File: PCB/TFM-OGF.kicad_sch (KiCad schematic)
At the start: 16 parts, among them J1 Alimentación, J2 CAN, J3 Jumper CAN, J4 Jumper CAN, U1 SN65HVD230, U2 SN65HVD230

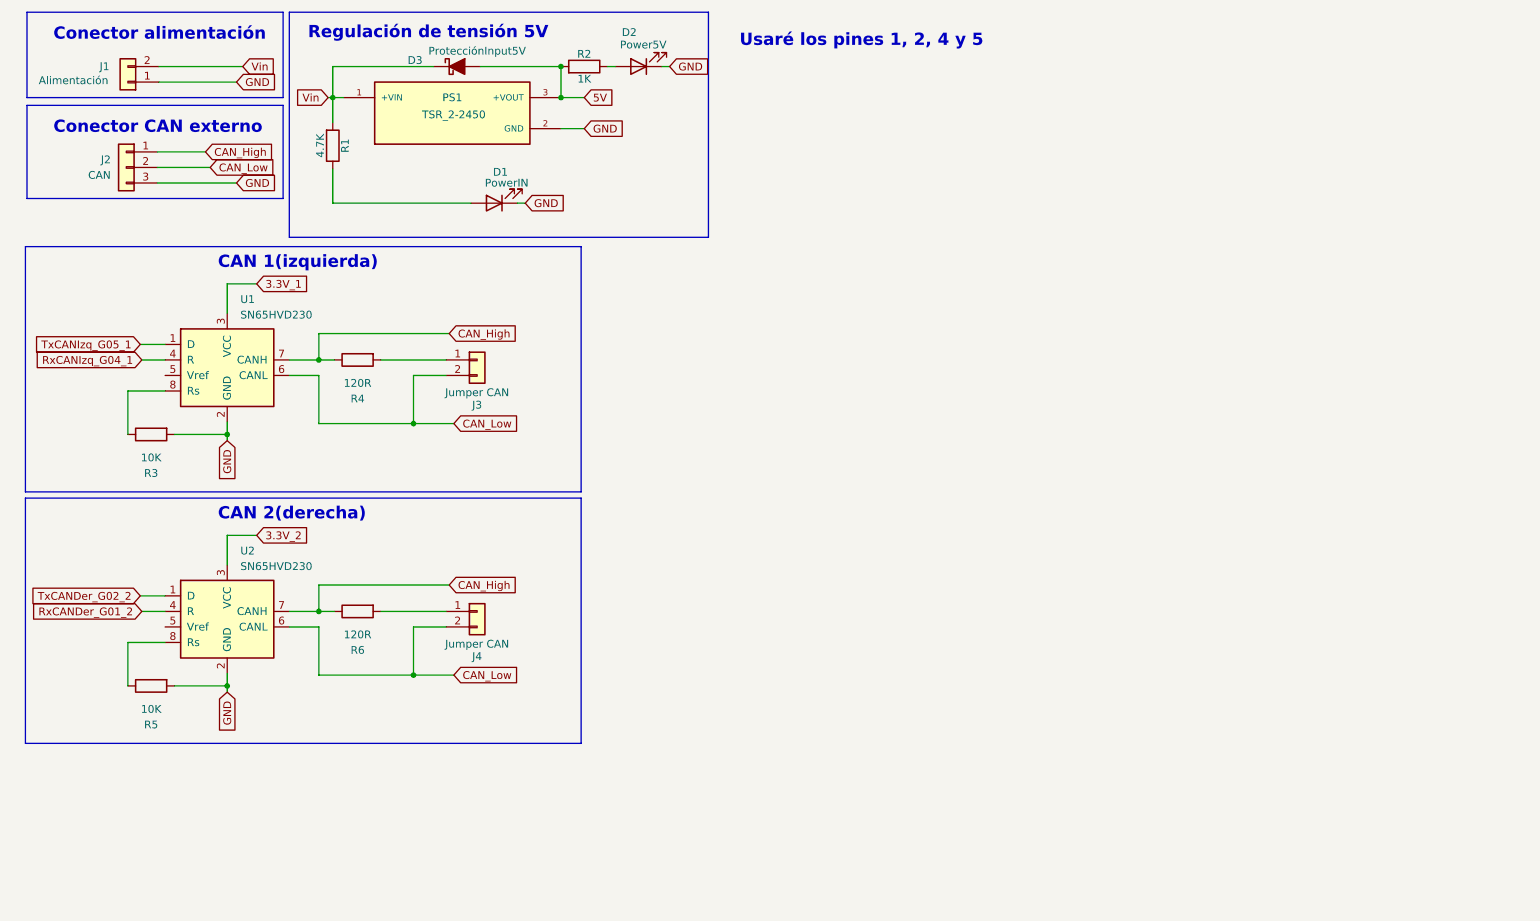
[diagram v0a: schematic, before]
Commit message: Finalizo esquemático, usaré medidas y caja de BrakeCAN
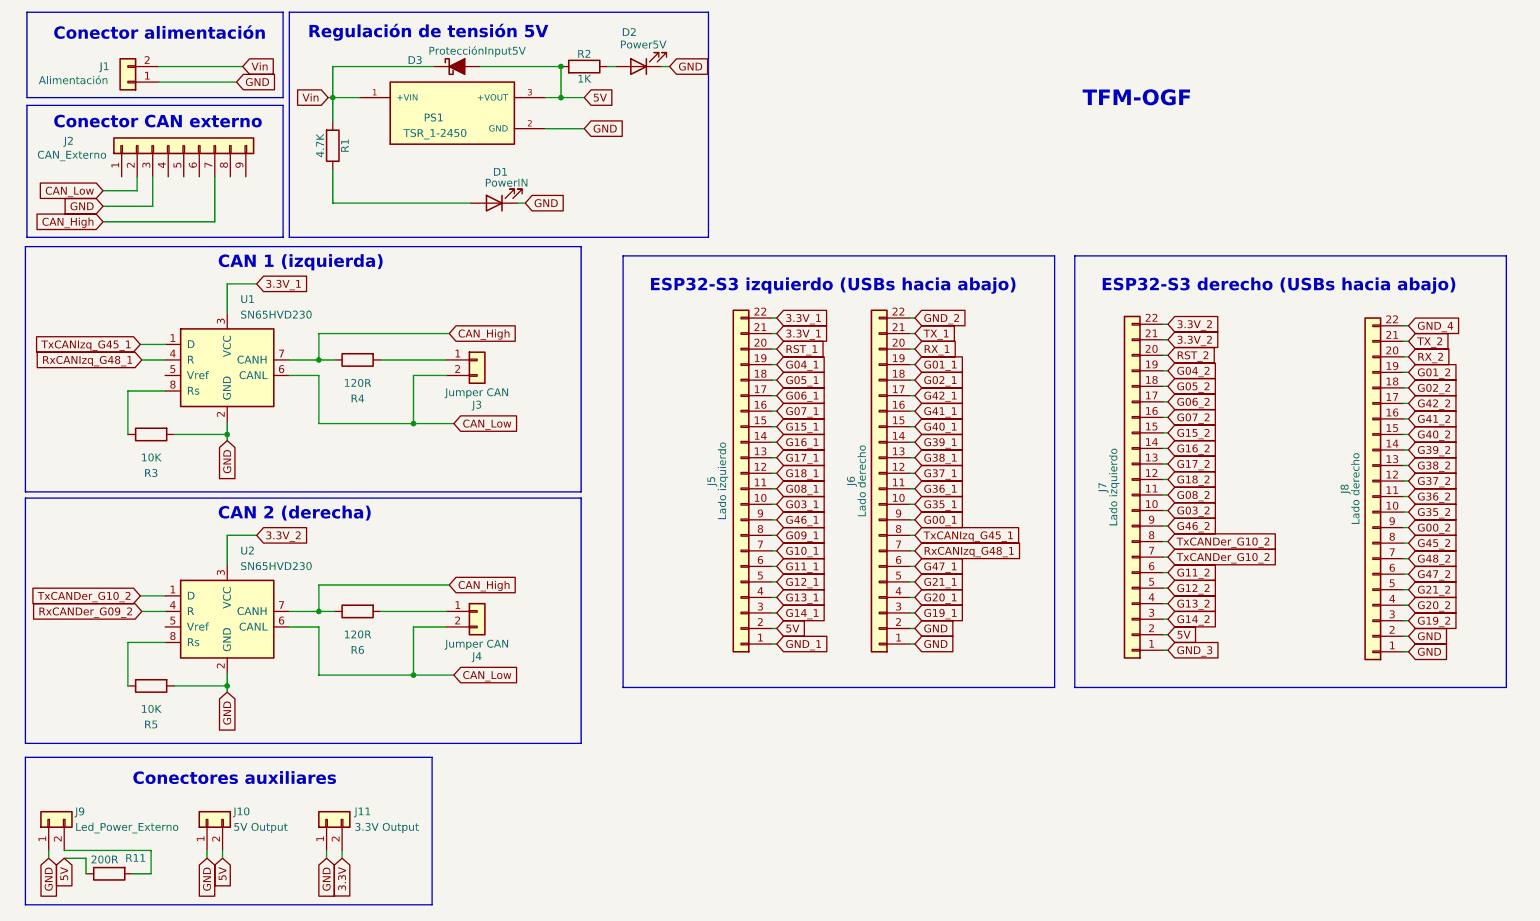
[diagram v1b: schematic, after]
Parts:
- removed J2: CAN, symbol Connector_Generic:Conn_01x03
- removed PS1: TSR_2-2450, TSR_2-2450:CONV_TSR_2-2450, symbol TSR_2-2450:TSR_2-2450
- added J10: 5V Output, Connector_JST:JST_XH_B2B-XH-A_1x02_P2.50mm_Vertical, symbol Connector_Generic:Conn_01x02
- added J11: 3.3V Output, Connector_JST:JST_XH_B2B-XH-A_1x02_P2.50mm_Vertical, symbol Connector_Generic:Conn_01x02
- added J2: CAN_Externo, Connector_Dsub:DSUB-9_Socket_Vertical_P2.77x2.84mm_MountingHoles, symbol Connector_Generic:Conn_01x09
- added J5, J7: Lado izquierdo, Connector_PinSocket_2.54mm:PinSocket_1x22_P2.54mm_Vertical, symbol Connector_Generic:Conn_01x22
- added J6, J8: Lado derecho, Connector_PinSocket_2.54mm:PinSocket_1x22_P2.54mm_Vertical, symbol Connector_Generic:Conn_01x22
- added J9: Led_Power_Externo, Connector_JST:JST_XH_B2B-XH-A_1x02_P2.50mm_Vertical, symbol Connector_Generic:Conn_01x02
- added PS1: TSR_1-2450, TSR_1-2450:CONV_TSR_1-2450, symbol TSR_1-2450:TSR_1-2450
- added R11: 200R, Resistor_SMD:R_0603_1608Metric, symbol Device:R
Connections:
- net 3.3V_1: now also J5.21 (Pin_21), J5.22 (Pin_22)
- net 3.3V_2: now also J7.21 (Pin_21), J7.22 (Pin_22)
- net 5V: now also J10.2 (Pin_2), J5.2 (Pin_2), J7.2 (Pin_2), PS1.3 (+VOUT), R11.1
- net CAN_High: now also J2.7 (Pin_7)
- net CAN_Low: now also J2.2 (Pin_2)
- net GND: now also J10.1 (Pin_1), J11.1 (Pin_1), J2.3 (Pin_3), J6.1 (Pin_1), J6.2 (Pin_2), J8.1 (Pin_1), J8.2 (Pin_2), J9.1 (Pin_1), PS1.2 (GND)
- net Vin: now also PS1.1 (+VIN)
- net RxCANDer_G01_2 renamed RxCANDer_G09_2
- net RxCANIzq_G04_1 renamed RxCANIzq_G48_1
- net RxCANIzq_G48_1: now also J6.7 (Pin_7)
- net TxCANDer_G02_2 renamed TxCANDer_G10_2
- net TxCANDer_G10_2: now also J7.7 (Pin_7), J7.8 (Pin_8)
- net TxCANIzq_G05_1 renamed TxCANIzq_G45_1
- net TxCANIzq_G45_1: now also J6.8 (Pin_8)
- new net: J9.2 (Pin_2), R11.2
- new net 3.3V: J11.2 (Pin_2)
- new net G00_1: J6.9 (Pin_9)
- new net G00_2: J8.9 (Pin_9)
- new net G01_1: J6.19 (Pin_19)
- new net G01_2: J8.19 (Pin_19)
- new net G02_1: J6.18 (Pin_18)
- new net G02_2: J8.18 (Pin_18)
- new net G03_1: J5.10 (Pin_10)
- new net G03_2: J7.10 (Pin_10)
- new net G04_1: J5.19 (Pin_19)
- new net G04_2: J7.19 (Pin_19)
- new net G05_1: J5.18 (Pin_18)
- new net G05_2: J7.18 (Pin_18)
- new net G06_1: J5.17 (Pin_17)
- new net G06_2: J7.17 (Pin_17)
- new net G07_1: J5.16 (Pin_16)
- new net G07_2: J7.16 (Pin_16)
- new net G08_1: J5.11 (Pin_11)
- new net G08_2: J7.11 (Pin_11)
- new net G09_1: J5.8 (Pin_8)
- new net G10_1: J5.7 (Pin_7)
- new net G11_1: J5.6 (Pin_6)
- new net G11_2: J7.6 (Pin_6)
- new net G12_1: J5.5 (Pin_5)
- new net G12_2: J7.5 (Pin_5)
- new net G13_1: J5.4 (Pin_4)
- new net G13_2: J7.4 (Pin_4)
- new net G14_1: J5.3 (Pin_3)
- new net G14_2: J7.3 (Pin_3)
- new net G15_1: J5.15 (Pin_15)
- new net G15_2: J7.15 (Pin_15)
- new net G16_1: J5.14 (Pin_14)
- new net G16_2: J7.14 (Pin_14)
- new net G17_1: J5.13 (Pin_13)
- new net G17_2: J7.13 (Pin_13)
- new net G18_1: J5.12 (Pin_12)
- new net G18_2: J7.12 (Pin_12)
- new net G19_1: J6.3 (Pin_3)
- new net G19_2: J8.3 (Pin_3)
- new net G20_1: J6.4 (Pin_4)
- new net G20_2: J8.4 (Pin_4)
- new net G21_1: J6.5 (Pin_5)
- new net G21_2: J8.5 (Pin_5)
- new net G35_1: J6.10 (Pin_10)
- new net G35_2: J8.10 (Pin_10)
- new net G36_1: J6.11 (Pin_11)
- new net G36_2: J8.11 (Pin_11)
- new net G37_1: J6.12 (Pin_12)
- new net G37_2: J8.12 (Pin_12)
- new net G38_1: J6.13 (Pin_13)
- new net G38_2: J8.13 (Pin_13)
- new net G39_1: J6.14 (Pin_14)
- new net G39_2: J8.14 (Pin_14)
- new net G40_1: J6.15 (Pin_15)
- new net G40_2: J8.15 (Pin_15)
- new net G41_1: J6.16 (Pin_16)
- new net G41_2: J8.16 (Pin_16)
- new net G42_1: J6.17 (Pin_17)
- new net G42_2: J8.17 (Pin_17)
- new net G45_2: J8.8 (Pin_8)
- new net G46_1: J5.9 (Pin_9)
- new net G46_2: J7.9 (Pin_9)
- new net G47_1: J6.6 (Pin_6)
- new net G47_2: J8.6 (Pin_6)
- new net G48_2: J8.7 (Pin_7)
- new net GND_1: J5.1 (Pin_1)
- new net GND_2: J6.22 (Pin_22)
- new net GND_3: J7.1 (Pin_1)
- new net GND_4: J8.22 (Pin_22)
- new net RST_1: J5.20 (Pin_20)
- new net RST_2: J7.20 (Pin_20)
- new net RX_1: J6.20 (Pin_20)
- new net RX_2: J8.20 (Pin_20)
- new net TX_1: J6.21 (Pin_21)
- new net TX_2: J8.21 (Pin_21)
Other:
- note added: "CAN 1 (izquierda)"
- note added: "CAN 2 (derecha)"
- note added: "Conectores auxiliares"
- note added: "ESP32-S3 derecho (USBs hacia abajo)"
- note added: "ESP32-S3 izquierdo (USBs hacia abajo)"
- note added: "TFM-OGF"
- note removed: "CAN 1(izquierda)"
- note removed: "CAN 2(derecha)"
- note removed: "Usaré los pines 1, 2, 4 y 5"
- company: (none) -> UNIR
- title: (none) -> TFM-OGF
